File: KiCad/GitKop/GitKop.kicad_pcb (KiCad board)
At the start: 2 copper layers, 58.5 x 126.5 mm, 35 parts, among them J1 POWER_Socket, J2 Conn_01x08_Socket, J3 Conn_01x04_Socket, J4 RJ45, Q1 BC557, Q2 BC547, Q3 IRF740, SW1 RotaryEncoder_Switch, U1 MCP6281, U2 TL071, U3 TL071, U4 LF33_TO252

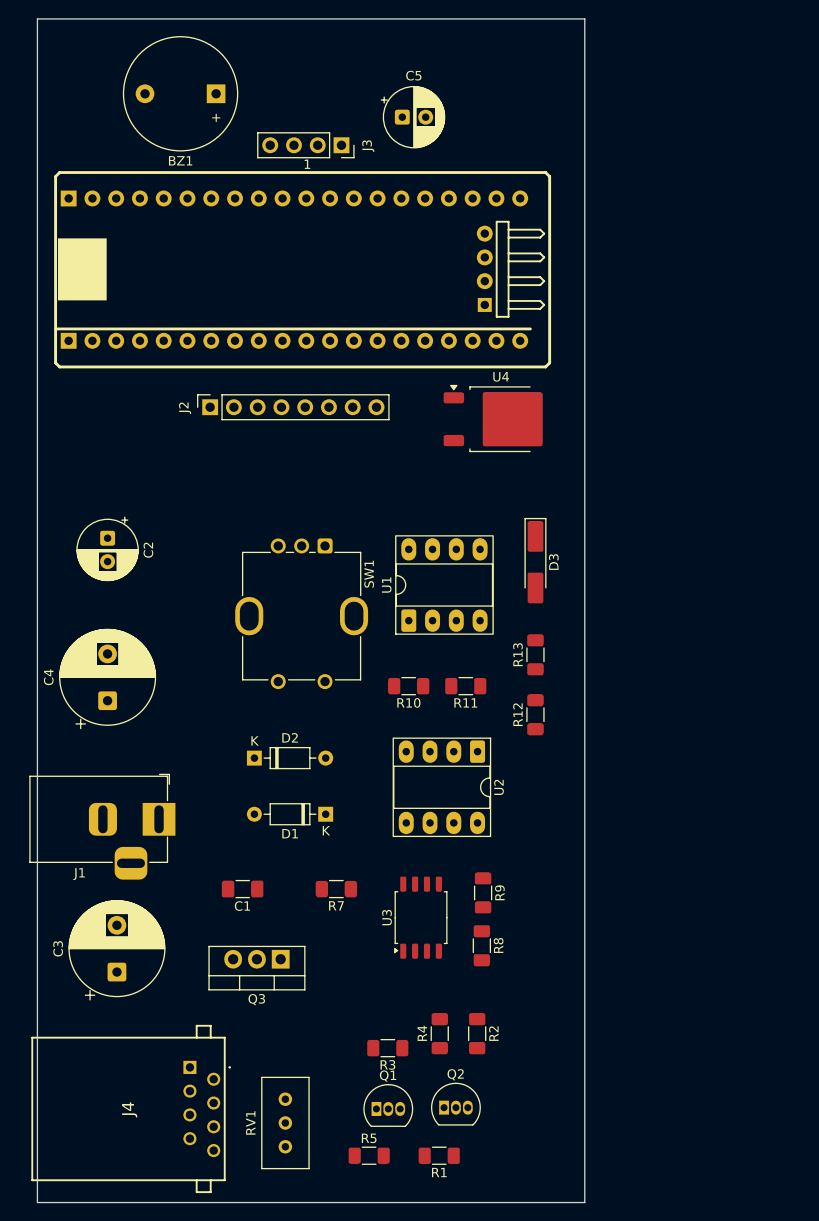
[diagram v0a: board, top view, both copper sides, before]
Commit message: gitkop001
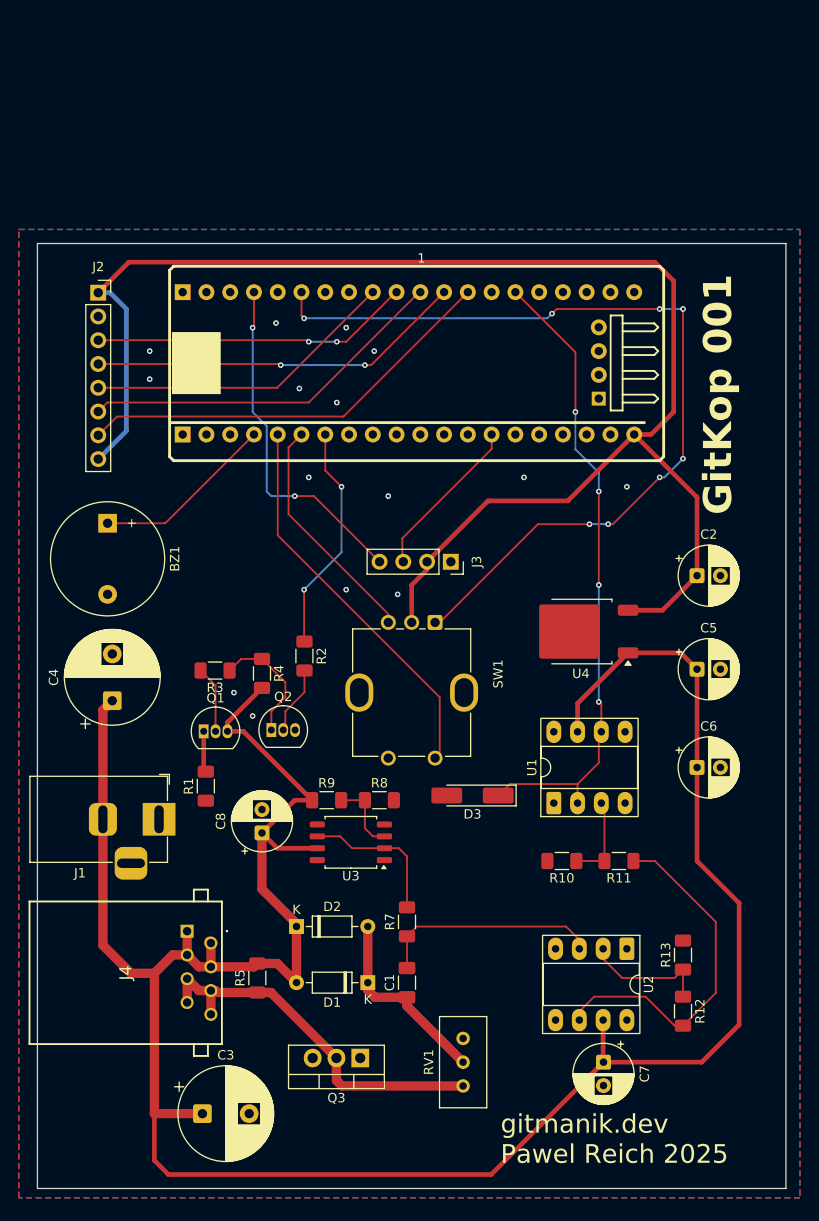
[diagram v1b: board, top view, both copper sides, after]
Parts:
- added C6: 100uF, Capacitor_THT:CP_Radial_D6.3mm_P2.50mm, F.Cu at (184.5, 125.0)
- added C7: 100uF, Capacitor_THT:CP_Radial_D6.3mm_P2.50mm, F.Cu at (174.5, 156.5)
- added C8: 100uF, Capacitor_THT:CP_Radial_D6.3mm_P2.50mm, F.Cu at (138.0, 132.0)
- moved C5 66.9 mm to (184.5, 114.5)
- moved C2 63.1 mm to (184.5, 104.5), turned to 0 degrees
- moved BZ1 47.3 mm to (121.5, 98.9), turned to -90 degrees
- moved R1 46.7 mm to (132.0, 127.0), turned to 90 degrees
- moved J3 46.0 mm to (158.2, 103.0)
- moved Q2 44.4 mm to (139.0, 121.0)
- moved Q1 44.4 mm to (131.8, 121.1)
- moved R2 44.4 mm to (142.5, 113.1)
- moved R3 44.4 mm to (133.0, 114.6)
- moved R4 42.9 mm to (138.0, 115.0), turned to -90 degrees
- moved R13 35.8 mm to (183.0, 145.1)
- moved R12 35.4 mm to (183.0, 151.1), turned to -90 degrees
- moved U2 26.4 mm to (177.0, 144.4)
- moved D3 25.8 mm to (160.5, 128.0), turned to 180 degrees
- moved U1 24.9 mm to (169.2, 128.8)
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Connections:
- 1 pad 10: BUZZER -> unconnected-(1A-PA15-Pad10)
- 1 pad 19: unconnected-(1A-GND-Pad19) -> GND
- 1 pad 31: LCD_DC -> LCD_CS
- 1 pad 32: unconnected-(1A-PA6-Pad32) -> LCD_DC
- 1 pad 4: unconnected-(1A-PB15-Pad4) -> BUZZER
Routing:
- net COIL2: track 0.00 -> 264.9 mm
- net 3_3V: track 0.00 -> 164.7 mm
- net ENC_A: track 0.00 -> 94.1 mm, vias 0 -> 8
- net SIGNAL_OUT: track 0.00 -> 68.5 mm, vias 0 -> 4
- net LCD_SCK: track 0.00 -> 45.8 mm
- net ENC_BTN: track 0.00 -> 42.0 mm
- net COIL1: track 0.00 -> 40.7 mm
- net LCD_RST: track 0.00 -> 40.2 mm, vias 0 -> 2
- net LCD_MOSI: track 0.00 -> 39.7 mm
- net Net-(R11-Pad1): track 0.00 -> 38.0 mm
- net I2C_SDA: track 0.00 -> 37.2 mm, vias 0 -> 2
- net LCD_CS: track 0.00 -> 34.1 mm, vias 0 -> 2
- net LCD_DC: track 0.00 -> 33.6 mm
- net ENC_B: track 0.00 -> 25.1 mm
- net PULSE_IN: track 0.00 -> 24.5 mm, vias 0 -> 2
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- added copper zone on B.Cu, net GND
- added copper zone on F.Cu, net GND
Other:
- board size 58.5 x 126.5 mm -> 80 x 101 mm
- board text added: "GitKop 001"
- board text added: "gitmanik.dev Pawel Reich 2025"
